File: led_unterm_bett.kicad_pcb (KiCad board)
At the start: 2 copper layers, 56 x 77 mm, 29 parts, among them J1 Conn_01x03, J2 Conn_01x03, J3 Conn_01x03, J4 Conn_01x02, J5 Screw_Terminal_01x02, J6 Conn_01x04, Q1 BSS138, Q2 BSS138, Q3 BSS138, U1 NodeMCU1.0(ESP-12E), U2 LM7805_TO220

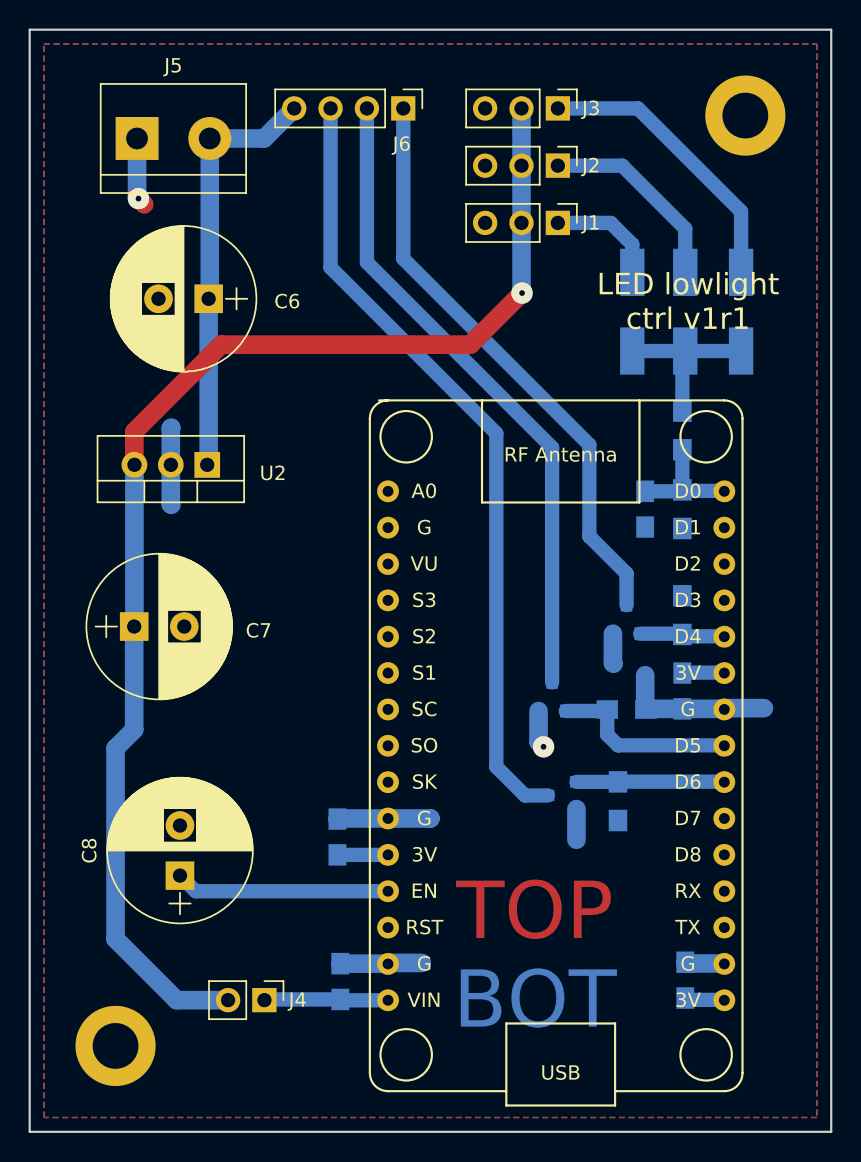
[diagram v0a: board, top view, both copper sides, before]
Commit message: migrate to kicad 6.0
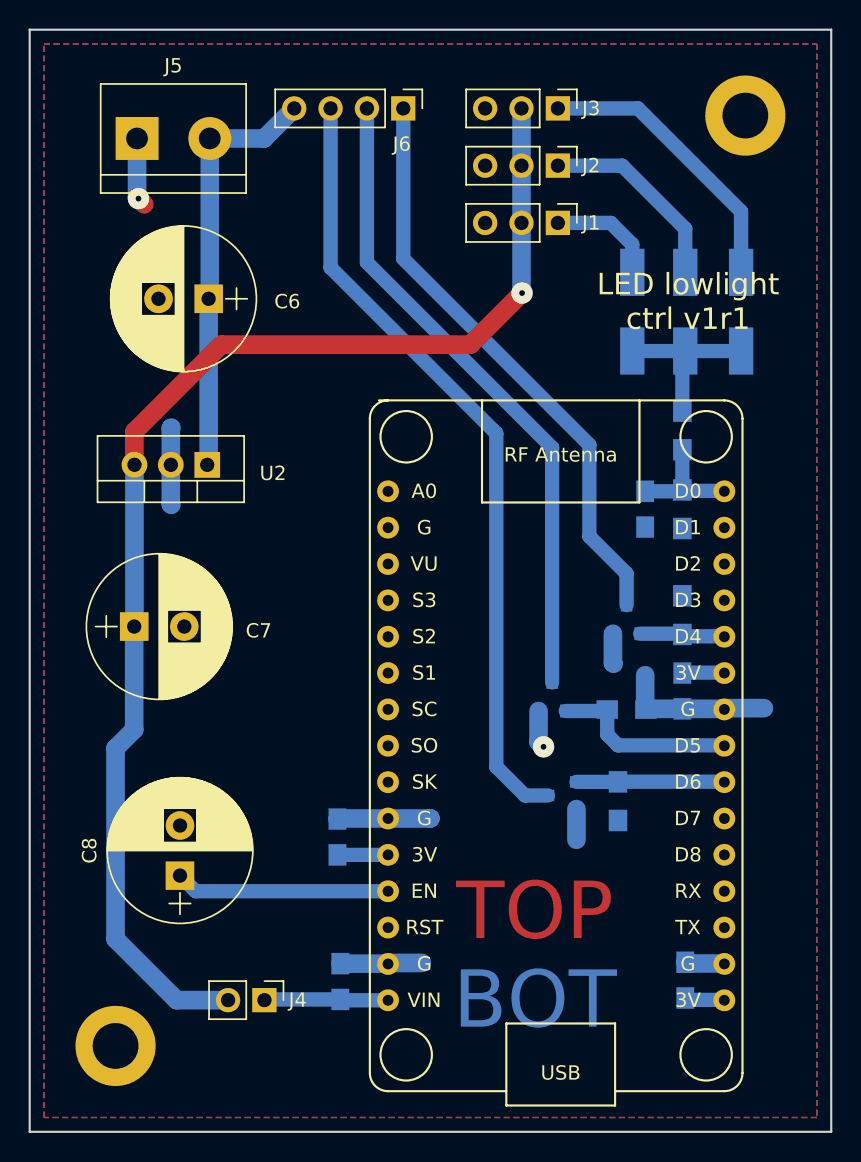
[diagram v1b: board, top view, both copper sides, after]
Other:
- net class Default removed
- net class Power removed
